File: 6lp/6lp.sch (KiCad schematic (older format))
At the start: 34 parts, among them J1 MODULE_HEADER, T1 2450BM15A0015, U1 AT86RF233, X1 16.0000MF09Z-AC3

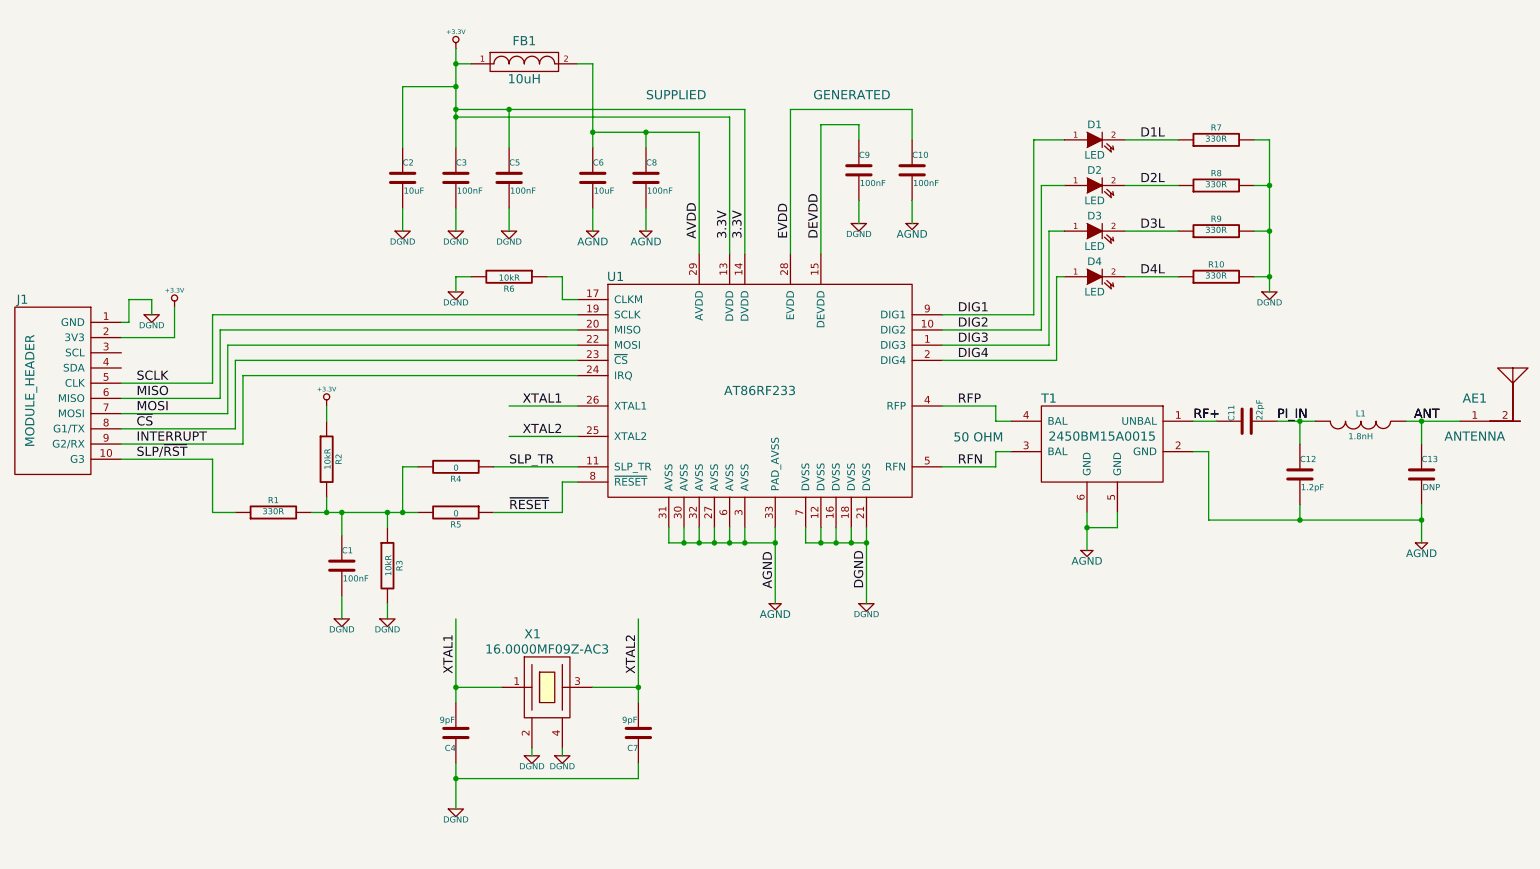
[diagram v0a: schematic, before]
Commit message: text, sch position tweaks
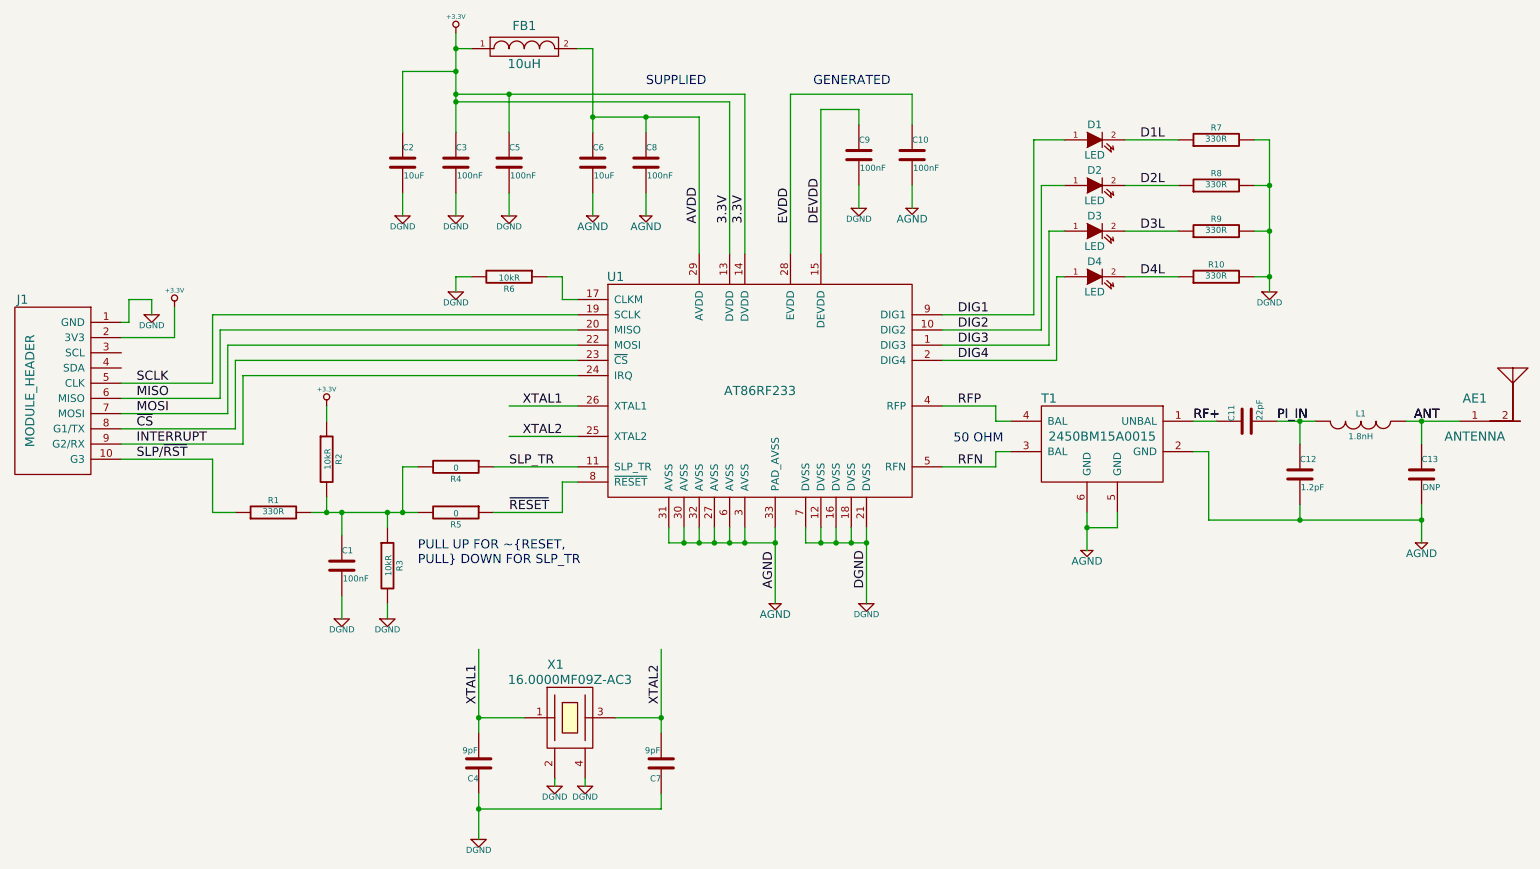
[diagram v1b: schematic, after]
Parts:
- X1: footprint (none) -> parts:TSX-3225
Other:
- note added: "PULL UP FOR ~RESET,\nPULL DOWN FOR SLP_TR"
- moved on the sheet: C10, C2, C3, C4, C5, C6, C7, C8, C9, FB1, X1
